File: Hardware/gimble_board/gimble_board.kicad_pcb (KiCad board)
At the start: 2 copper layers, 101 parts, among them J1 Test_Point, J2 Test_Point, J3 Test_Point, J4 Test_Point, Q1 Q_NMOS_GDS, Q2 Q_NMOS_GDS, Q3 Q_NMOS_GDS, Q4 Q_NMOS_GDS, Q5 Q_NMOS_GDS, Q6 Q_NMOS_GDS, Q7 Q_NMOS_GDS, Q8 Q_NMOS_GDS, SW1 SW_Push, SW2 SW_Push, SW3 SW_Push, SW4 SW_Push, SW5 SW_Push, SW6 SW_Push, SW7 SW_Push, SW8 SW_Push, SW9 SW_SPDT, U1 LM2576SX-3.3, U2 LM2576SX-5.0, U3 TM4C129E_Launchpad

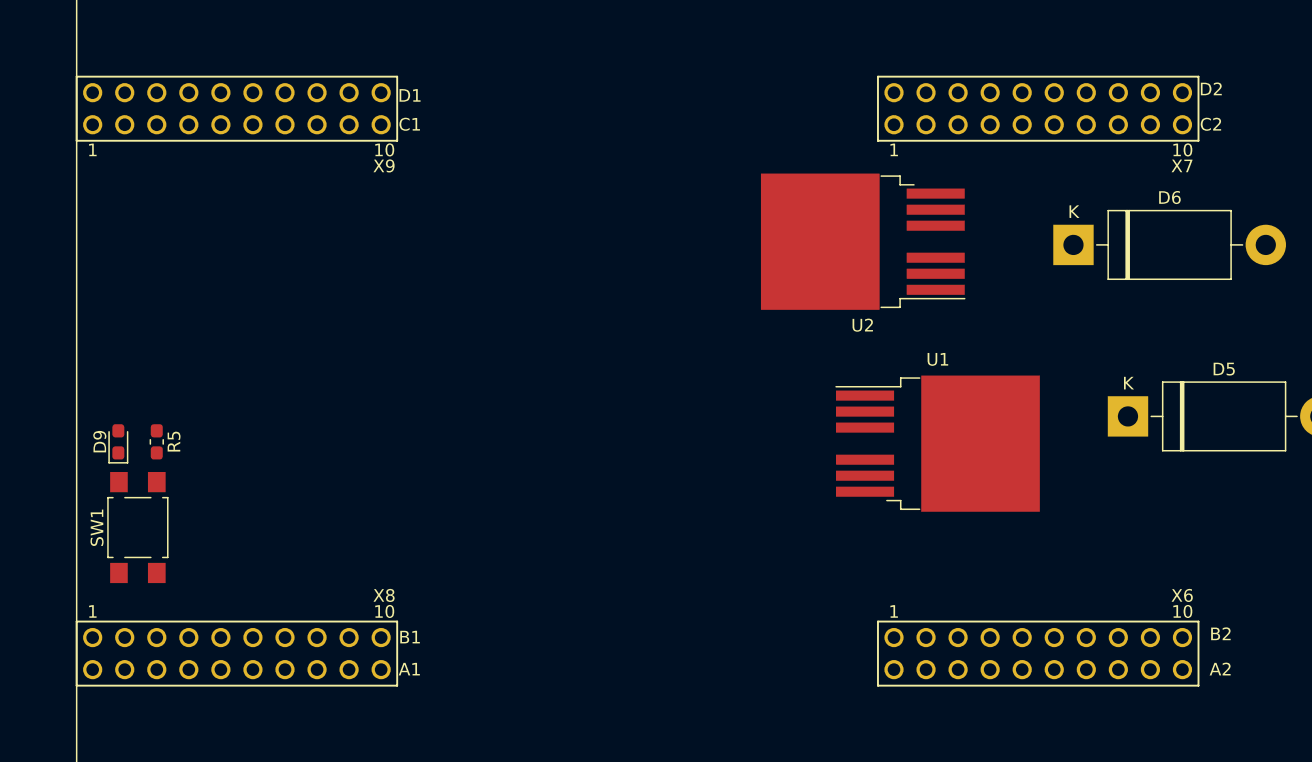
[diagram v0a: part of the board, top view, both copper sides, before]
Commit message: layout 3
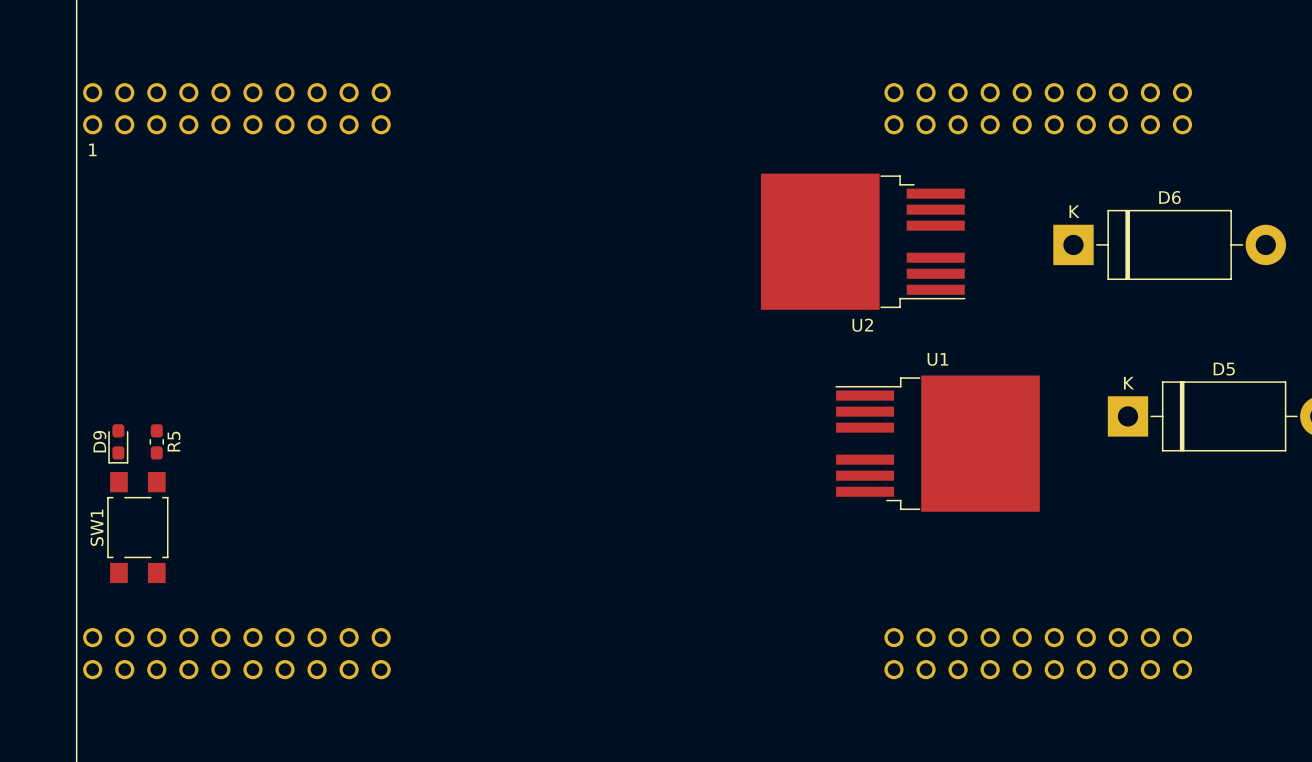
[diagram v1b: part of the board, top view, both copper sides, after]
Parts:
- U3: footprint MRDT_Shields:TM4C129E_Launchpad_FULL_THT_TOP -> MRDT_Shields:TM4C129E_Launchpad_FULL_THT_BOTTOM
